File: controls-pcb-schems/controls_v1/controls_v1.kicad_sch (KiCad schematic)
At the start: 13 parts, among them J1 Raspberry_Pi_4, U2 MS5607-02BA, U3 DRV5053EAQLPG

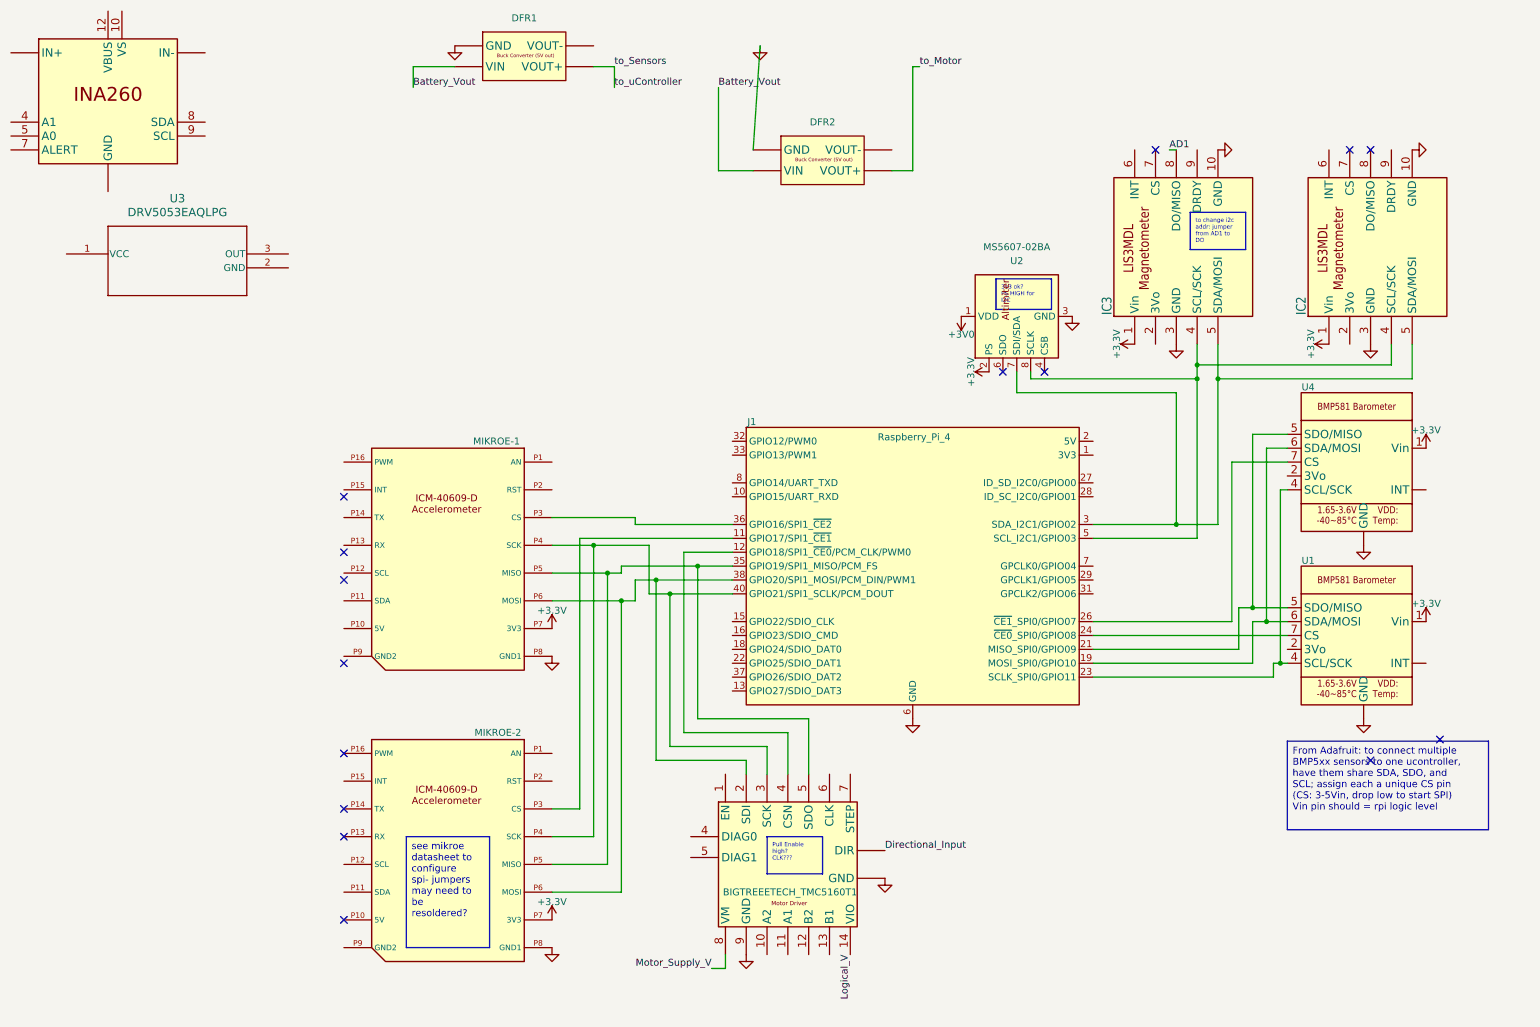
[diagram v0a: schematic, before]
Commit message: more schematic wiring updates
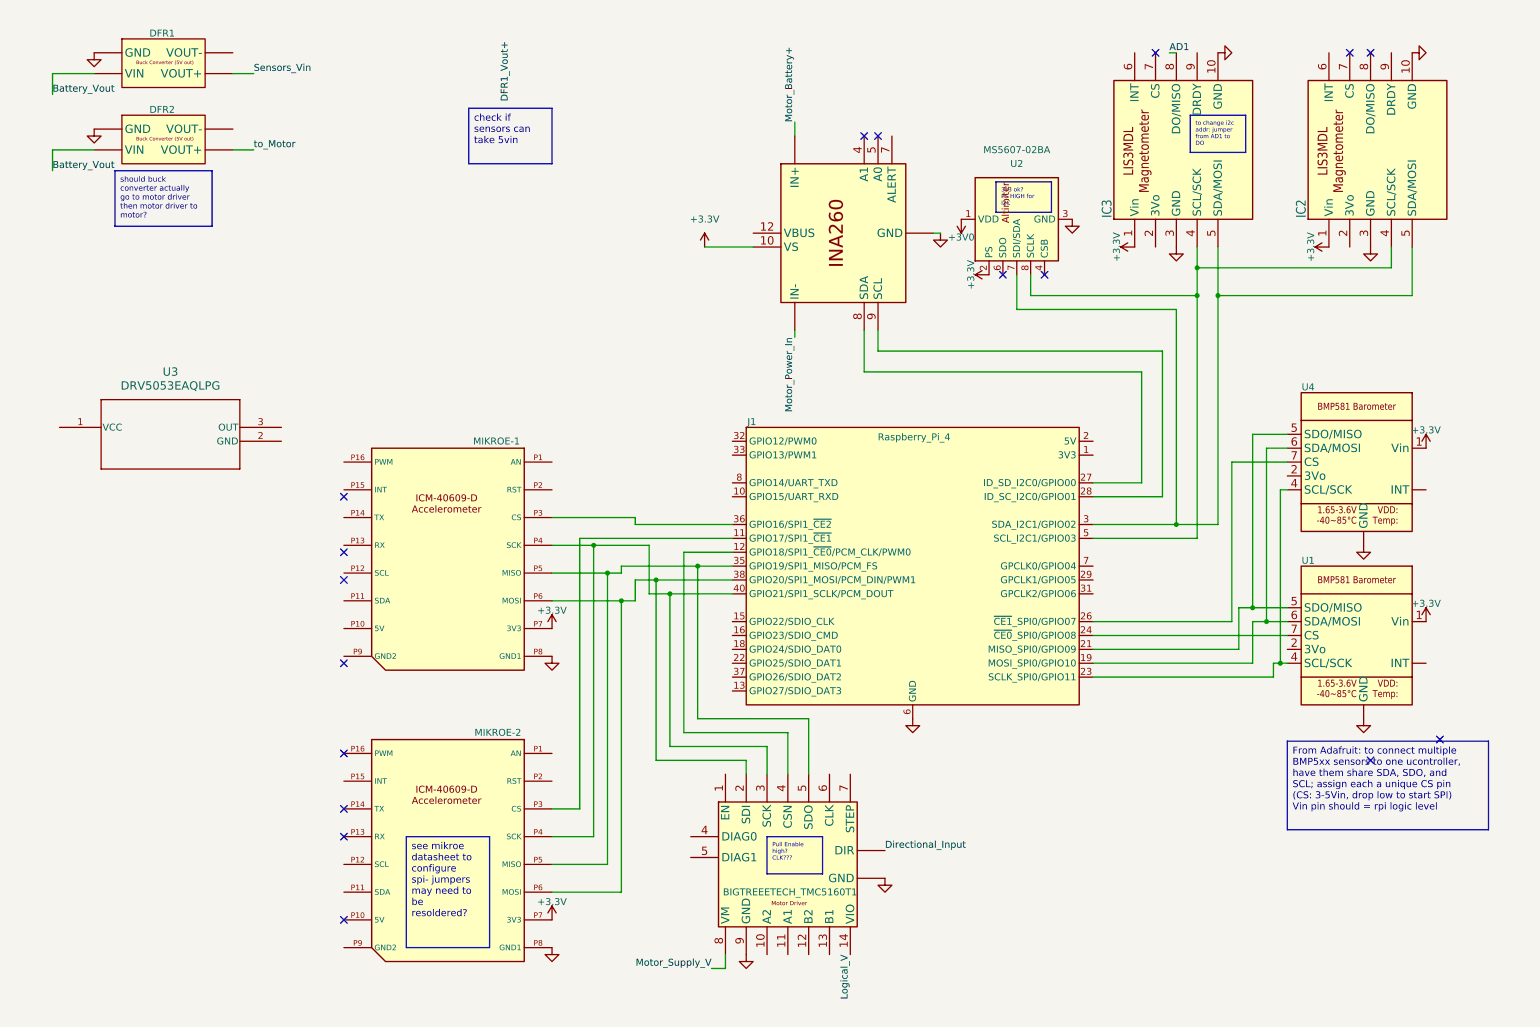
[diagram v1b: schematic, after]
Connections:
- net to_Sensors is gone; now on net Sensors_Vin: DFR1. (VOUT+)
- net +3.3V: now also IC1.10 (VS)
- net GND: now also IC1.11 (GND), IC1.13 (GND), IC1.6 (GND)
- net at BIGTREEETECH_TMC5160T1.4 (DIAG0): now also J1.12 (GPIO18/SPI1_~{CE0}/PCM_CLK/PWM0)
- net at BIGTREEETECH_TMC5160T1.5 (DIAG1): now also J1.35 (GPIO19/SPI1_MISO/PCM_FS), MIKROE-1.P5 (MISO), MIKROE-2.P5 (MISO)
- net Sensors_Vin: now reaches DFR1. (VOUT+)
- net at J1.27 (ID_SD_I2C0/GPIO00): now also IC1.8 (SDA)
- net at J1.28 (ID_SC_I2C0/GPIO01): now also IC1.9 (SCL)
- net Motor_Battery+: now reaches IC1.1 (IN+), IC1.2 (IN+), IC1.3 (IN+)
- net Motor_Power_In: now reaches IC1.14 (IN-), IC1.15 (IN-), IC1.16 (IN-)
- no-connect marks 15 -> 17
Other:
- moved on the sheet: DFR1, DFR2, IC2, IC3, U2, U3
